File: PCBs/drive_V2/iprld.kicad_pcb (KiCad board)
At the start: 2 copper layers, 100 x 100 mm, 87 parts, among them IC1 W25Q16JVUXIQ_TR, IC2 ADS1115IDGSR, J1 TYPE-C-31-M-12, U1 AMS1117-3.3, U11 4N35, U12 4N35, U13 4N35, U14 4N35, U2 ESP32-S3, U3 4N35, U4 USBLC6-4SC6, U5 TCA9548APWR, U6 4N35, U7 4N35, U8 4N35, U9 AMS1117-5.0, Y1 7M40000010

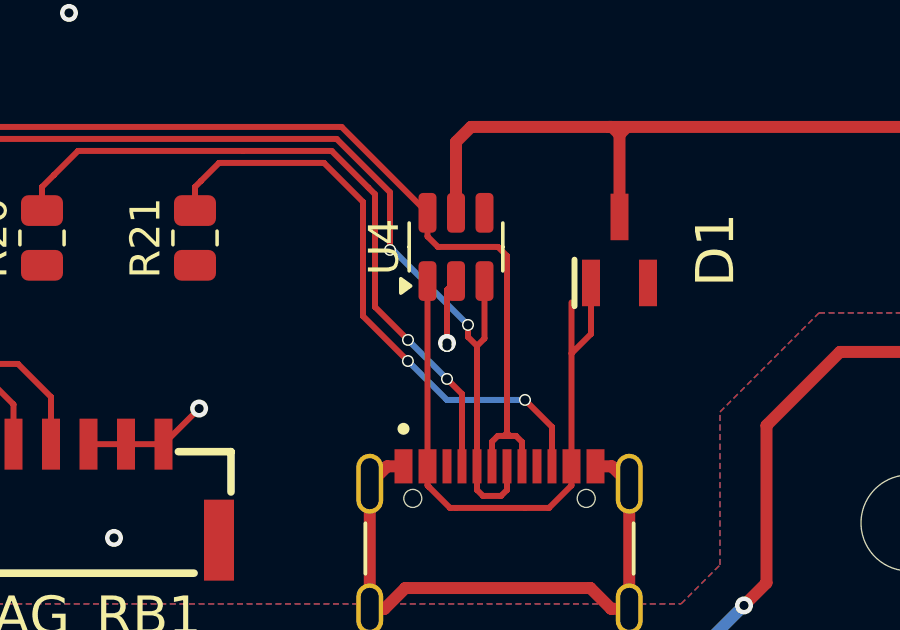
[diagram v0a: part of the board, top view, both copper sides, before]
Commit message: fixed merge issues
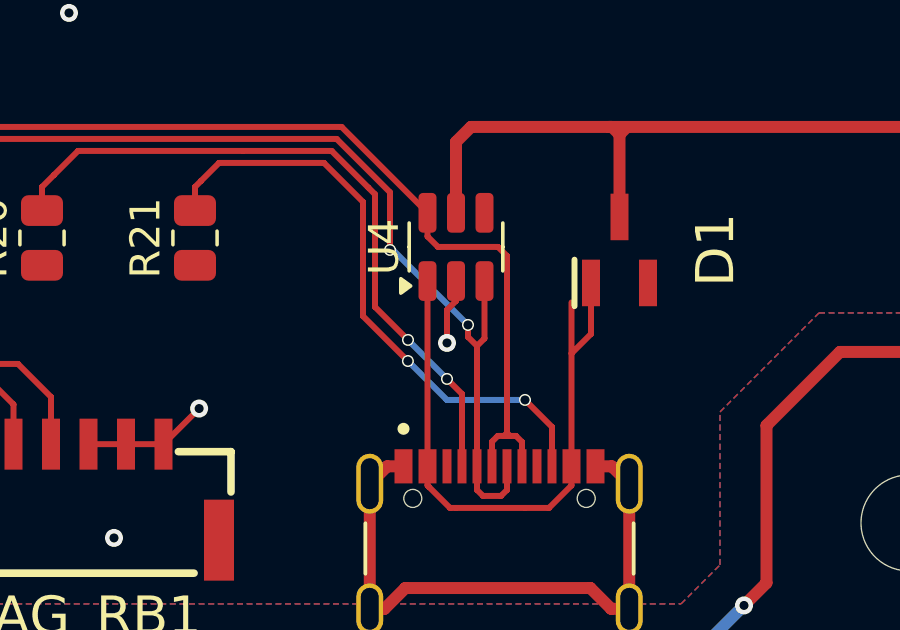
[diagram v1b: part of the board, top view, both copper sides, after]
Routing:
- net GND: track 251.2 -> 248.9 mm, vias 45 -> 44
